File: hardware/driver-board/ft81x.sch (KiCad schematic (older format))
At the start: 5 parts, among them U6 FT813, X1 YSX321SL

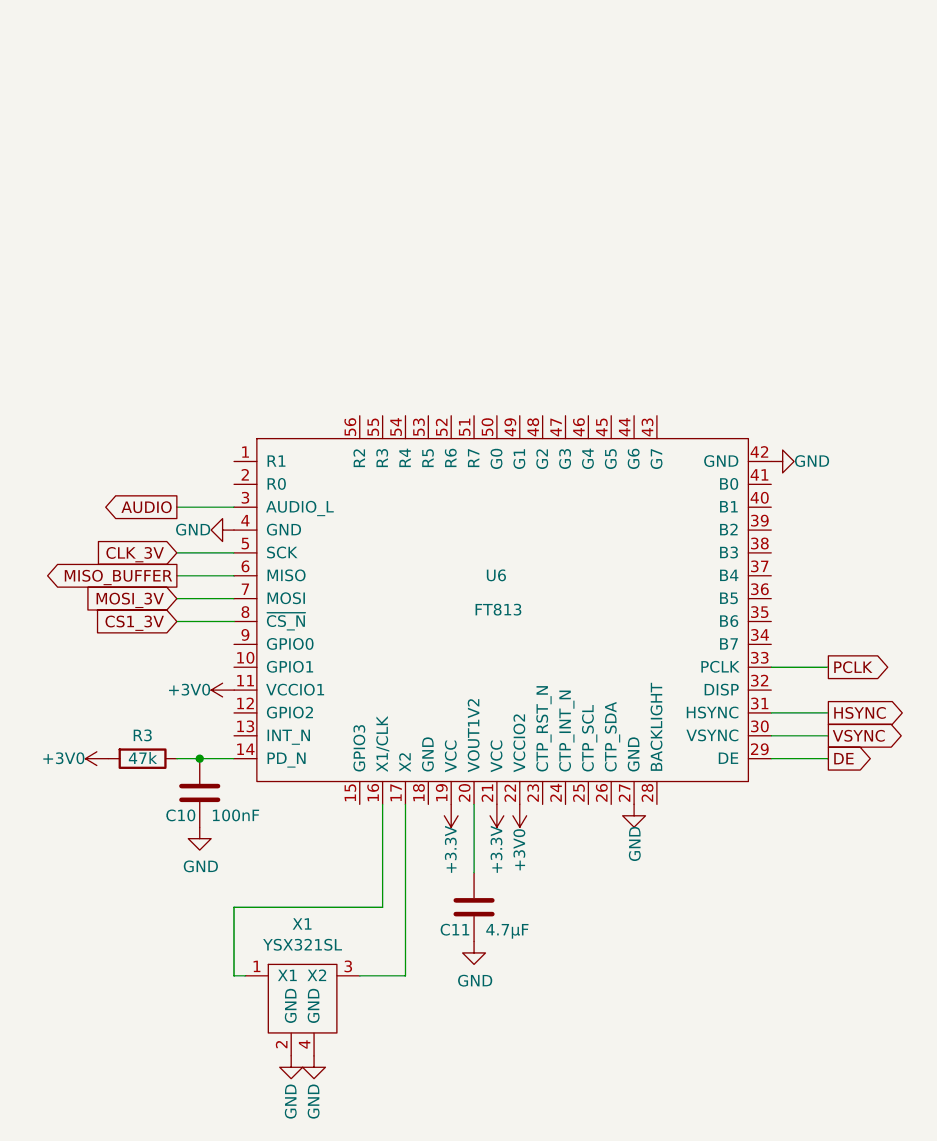
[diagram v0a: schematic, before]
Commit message: Add display schematics
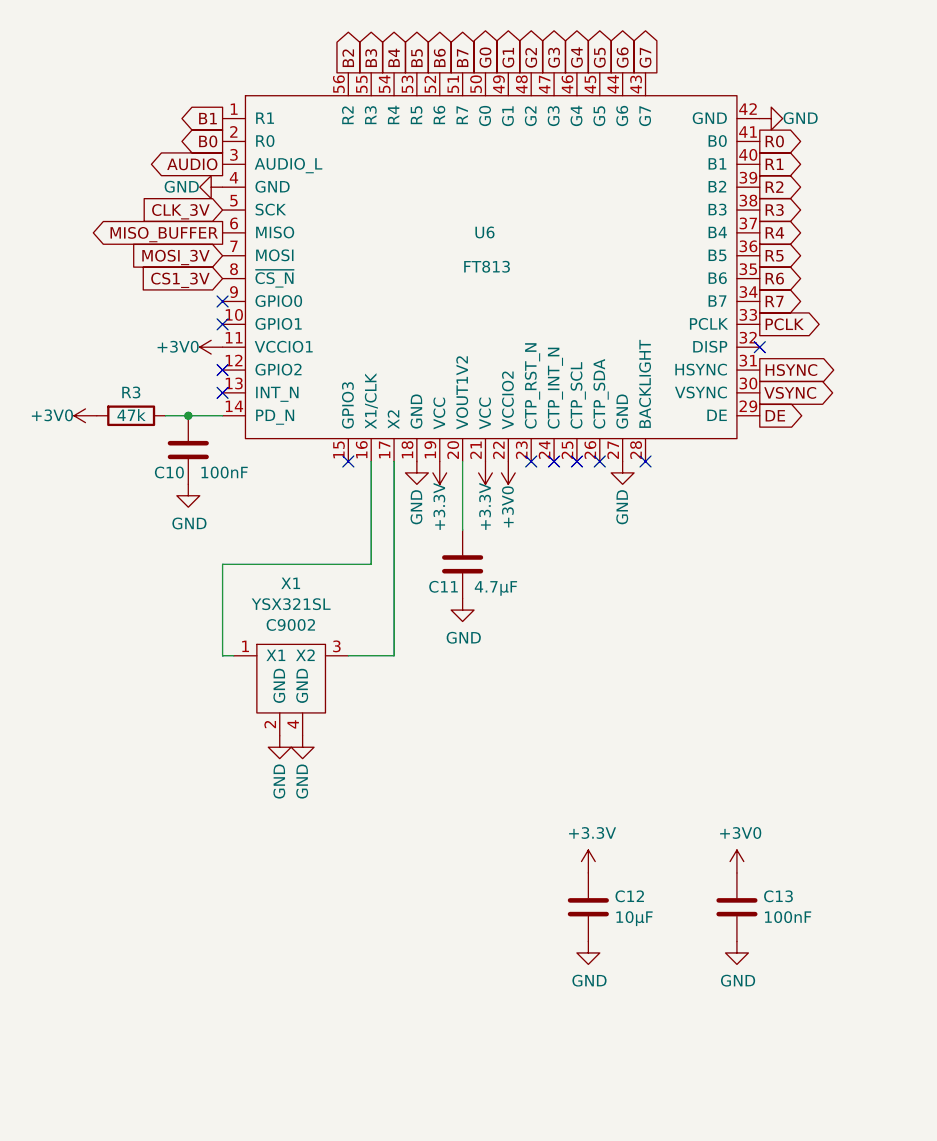
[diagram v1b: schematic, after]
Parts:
- added C12: 10µF, Capacitor_SMD:C_0603_1608Metric, symbol Device:C
- added C13: 100nF, Capacitor_SMD:C_0603_1608Metric, symbol Device:C
- X1: JLCPCB (none) -> C9002
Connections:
- net +3V0: now also C13.1
- net +3V3: now also C12.1
- net GND: now also U6.18 (GND), C12.2, C13.2
- net B1: now reaches U6.1 (R1)
- net B0: now reaches U6.2 (R0)
- net R7: now reaches U6.34 (B7)
- net R6: now reaches U6.35 (B6)
- net R5: now reaches U6.36 (B5)
- net R4: now reaches U6.37 (B4)
- net R3: now reaches U6.38 (B3)
- net R2: now reaches U6.39 (B2)
- net R1: now reaches U6.40 (B1)
- net R0: now reaches U6.41 (B0)
- net G7: now reaches U6.43 (G7)
- net G6: now reaches U6.44 (G6)
- net G5: now reaches U6.45 (G5)
- net G4: now reaches U6.46 (G4)
- net G3: now reaches U6.47 (G3)
- net G2: now reaches U6.48 (G2)
- net G1: now reaches U6.49 (G1)
- net G0: now reaches U6.50 (G0)
- net B7: now reaches U6.51 (R7)
- net B6: now reaches U6.52 (R6)
- net B5: now reaches U6.53 (R5)
- net B4: now reaches U6.54 (R4)
- net B3: now reaches U6.55 (R3)
- net B2: now reaches U6.56 (R2)
- no-connect marks 0 -> 11
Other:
- moved on the sheet: C10, C11, R3, U6, X1
